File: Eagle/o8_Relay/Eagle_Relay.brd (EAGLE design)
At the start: 40 x 21.9 mm, 9 parts, among them Q1 S9013, U1 HLS8L-DC3V-S-C

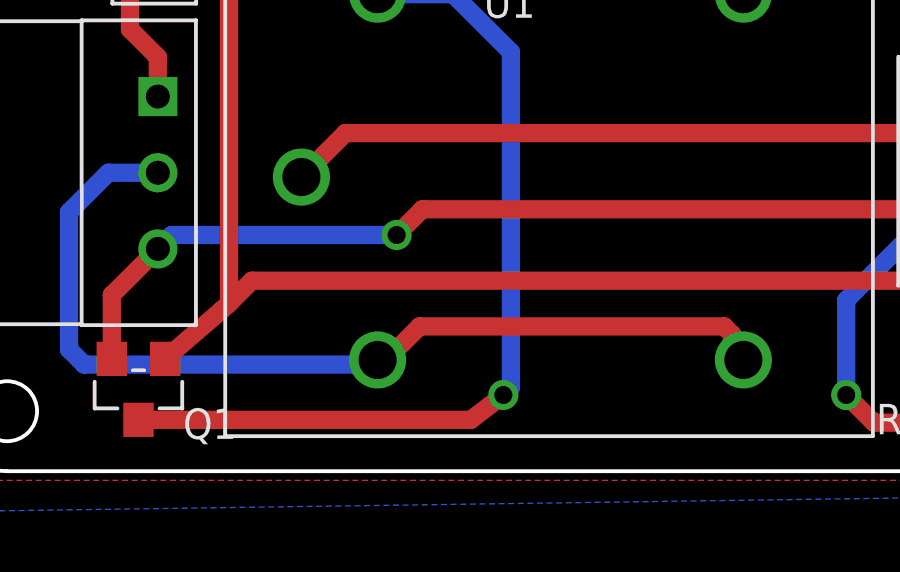
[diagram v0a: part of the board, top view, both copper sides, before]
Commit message: miniuno
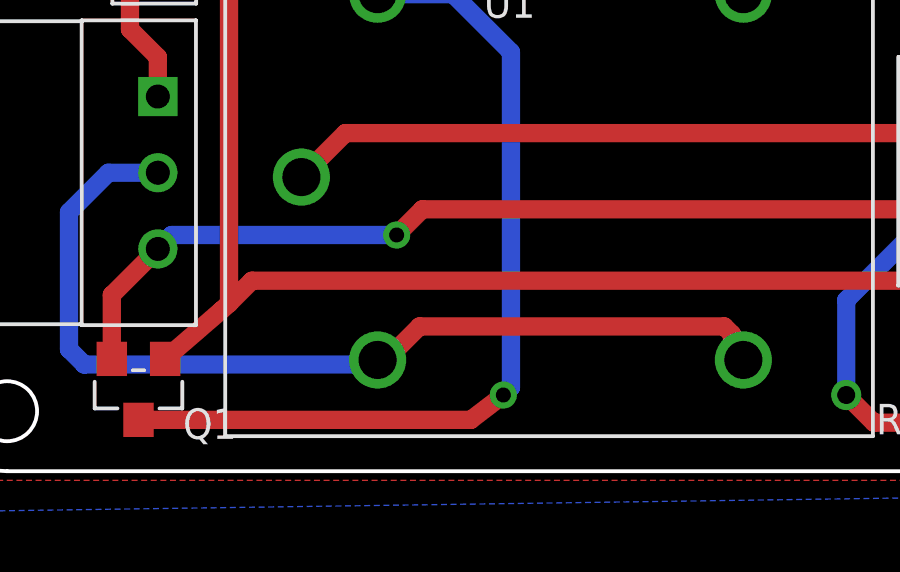
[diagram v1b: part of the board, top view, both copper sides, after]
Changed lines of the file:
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@@
 <setting verticaltext="up"/>
 </settings>
-<grid distance="10" unitdist="mil" unit="mm" style="lines" multiple="1" display="yes" altdistance="0.025" altunitdist="inch" altunit="inch"/>
+<grid distance="10" unitdist="mil" unit="mil" style="lines" multiple="1" display="yes" altdistance="0.025" altunitdist="inch" altunit="inch"/>
 <layers>
 <layer number="1" name="Top" color="4" fill="1" visible="yes" active="yes"/>
@@
 <wire x1="33.2714" y1="1.6176" x2="30.8944" y2="1.6176" width="0.6096" layer="1"/>
 <wire x1="30.8944" y1="1.6176" x2="29.972" y2="2.54" width="0.6096" layer="1"/>
-<via x="29.972" y="2.54" extent="1-16" drill="0.6" shape="square"/>
+<via x="29.972" y="2.54" extent="1-16" drill="0.6"/>
 <wire x1="29.972" y1="2.54" x2="29.972" y2="5.702" width="0.6096" layer="16"/>
 <wire x1="29.972" y1="5.702" x2="33" y2="8.73" width="0.6096" layer="16"/>
 <wire x1="33" y1="8.73" x2="15.842" y2="8.73" width="0.6096" layer="1"/>
 <wire x1="15.842" y1="8.73" x2="14.986" y2="7.874" width="0.6096" layer="1"/>
-<via x="14.986" y="7.874" extent="1-16" drill="0.6" shape="square"/>
+<via x="14.986" y="7.874" extent="1-16" drill="0.5"/>
 <wire x1="14.986" y1="7.874" x2="7.4902" y2="7.874" width="0.6096" layer="16"/>
 <wire x1="7.4902" y1="7.874" x2="7.0254" y2="7.4092" width="0.6096" layer="16"/>
@@
 <wire x1="6.38" y1="1.712" x2="17.46" y2="1.712" width="0.6096" layer="1"/>
 <wire x1="17.46" y1="1.712" x2="18.542" y2="2.54" width="0.6096" layer="1"/>
-<via x="18.542" y="2.54" extent="1-16" drill="0.6" shape="square"/>
+<via x="18.542" y="2.54" extent="1-16" drill="0.5"/>
 <wire x1="18.542" y1="2.54" x2="18.796" y2="2.794" width="0.6096" layer="16"/>
 </signal>
